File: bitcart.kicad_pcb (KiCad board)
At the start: 4 copper layers, 110 x 100 mm, 125 parts, among them J1 USB_OTG, J10 Conn_02x03_Odd_Even, J12 0455580003, J13 Hashboard0, J14 Hashboard1, J15 Hashboard2, J16 0353180420, J17 0353180420, J18 0353180420, J19 0353180420, J2 690-008-221-904, J3 61900411021, J4 61900411021, J5 61900411021, J6 61900411021, J7 Conn_01x22, J8 Conn_01x02, J9 THD-20-R, Q1 DMP3013SFV-7, U1 FSUSB42MUX, U10 PCA9546ARGVR, U2 USB2514B-I/M2, U3 TPD4EUSB30, U4 AP22653W6, U5 EMC2305-1-AP-TR, U6 74LVC1G07SE-7, U7 MagJack-A70-112-331N126, U9 AP64501SP-13, Y1 24MHz

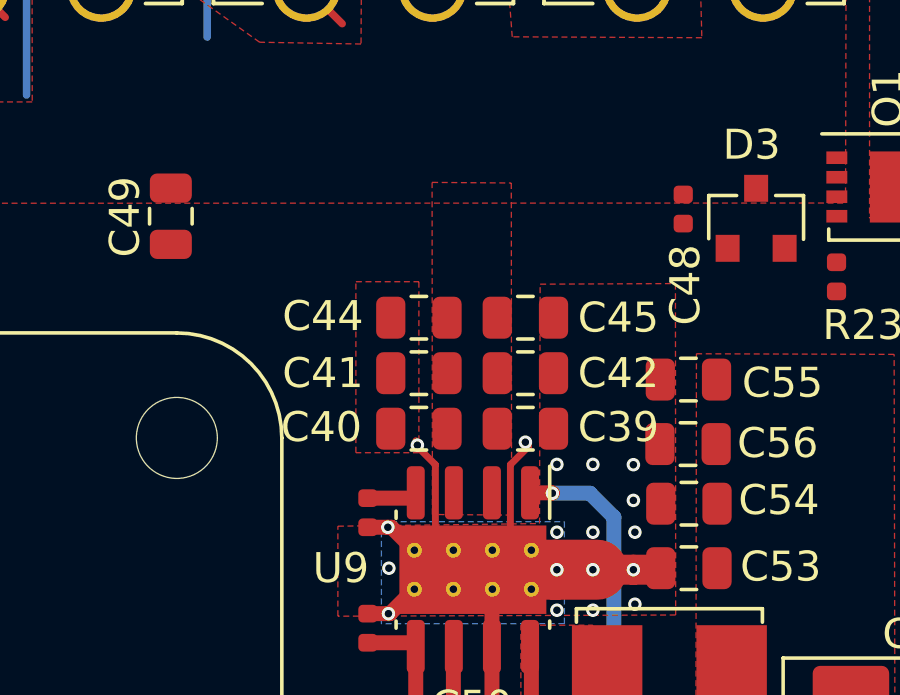
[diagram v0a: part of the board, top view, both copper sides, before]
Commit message: more placement
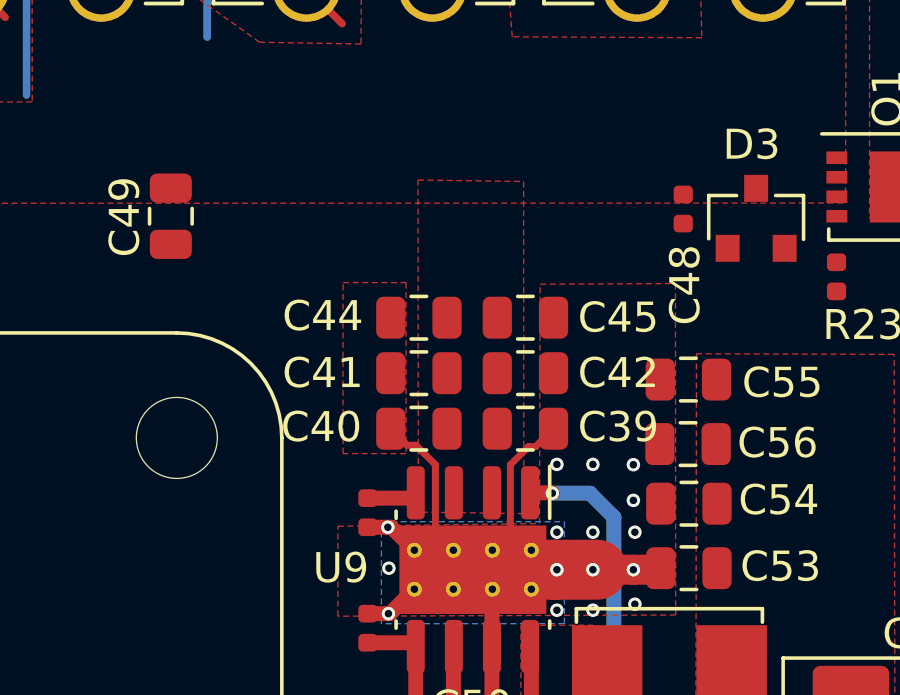
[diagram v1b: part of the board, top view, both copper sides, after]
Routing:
- net GND: track 172.9 -> 174.7 mm, vias 208 -> 206
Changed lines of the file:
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@@
   (segment (start 124.47 108.5) (end 124.47 107.8) (width 0.2) (layer "F.Cu") (net 1))
   (segment (start 117.27 105.4) (end 117.27 104.71001) (width 0.2) (layer "F.Cu") (net 1))
+  (segment (start 157.688553 73.792422) (end 157.926053 73.792422) (width 0.23) (layer "F.Cu") (net 1))
   (segment (start 116.07 105.42) (end 116.07 106.1) (width 0.2) (layer "F.Cu") (net 1))
   (segment (start 113.09 39.66) (end 114.1975 39.66) (width 0.25) (layer "F.Cu") (net 1))
-  (segment (start 153.938553 73.592422) (end 153.938553 73.742422) (width 0.23) (layer "F.Cu") (net 1))
   (segment (start 122.07 107.81001) (end 122.08001 107.8) (width 0.2) (layer "F.Cu") (net 1))
   (segment (start 157.088553 74.392422) (end 157.088553 76.642422) (width 0.23) (layer "F.Cu") (net 1))
@@
   (segment (start 171.054 109.294) (end 171.485 109.725) (width 0.5) (layer "F.Cu") (net 1))
   (segment (start 175.914 114.818) (end 175.914 112.729) (width 0.5) (layer "F.Cu") (net 1))
+  (segment (start 153.651053 73.742422) (end 153.101053 73.192422) (width 0.23) (layer "F.Cu") (net 1))
   (segment (start 125.27 74.58) (end 125.27 75.1) (width 0.2) (layer "F.Cu") (net 1))
   (segment (start 116.47 72.11137) (end 116.406823 72.174547) (width 0.2) (layer "F.Cu") (net 1))
@@
   (segment (start 120.87 108.5) (end 120.87 108.35) (width 0.2) (layer "F.Cu") (net 1))
   (segment (start 119.27 74.58) (end 119.27 75.4) (width 0.2) (layer "F.Cu") (net 1))
-  (segment (start 157.688553 73.592422) (end 157.688553 73.792422) (width 0.23) (layer "F.Cu") (net 1))
   (segment (start 125.27 74.58) (end 125.27 73.980058) (width 0.2) (layer "F.Cu") (net 1))
   (segment (start 179.635 108.575) (end 179.635 108.0375) (width 0.5) (layer "F.Cu") (net 1))
@@
   (segment (start 175.914 114.818) (end 177.91 116.814) (width 0.5) (layer "F.Cu") (net 1))
   (segment (start 178.31 119.95) (end 177.91 120.35) (width 0.2) (layer "F.Cu") (net 1))
+  (segment (start 157.926053 73.792422) (end 158.526053 73.192422) (width 0.23) (layer "F.Cu") (net 1))
   (segment (start 170.9505 109.294) (end 170.9505 110.214474) (width 1) (layer "F.Cu") (net 1))
   (segment (start 178.31 119.55) (end 178.31 119.95) (width 0.2) (layer "F.Cu") (net 1))
@@
   (segment (start 124.45999 105.41001) (end 124.45999 106.1) (width 0.2) (layer "F.Cu") (net 1))
   (segment (start 114.87 108.5) (end 114.87 107.8) (width 0.2) (layer "F.Cu") (net 1))
+  (segment (start 153.938553 73.742422) (end 153.651053 73.742422) (width 0.23) (layer "F.Cu") (net 1))
   (segment (start 120.87 107.8) (end 120.77 107.7) (width 0.13) (layer "F.Cu") (net 1))
   (segment (start 128.07 74.58) (end 128.07 73.9) (width 0.2) (layer "F.Cu") (net 1))
@@
   (via (at 126.88001 104.699345) (size 0.45) (drill 0.25) (layers "F.Cu" "B.Cu") (net 1))
   (via (at 186.2 43.985) (size 0.8) (drill 0.4) (layers "F.Cu" "B.Cu") (free) (net 1))
-  (via (at 157.588553 73.642422) (size 0.45) (drill 0.25) (layers "F.Cu" "B.Cu") (net 1))
   (via (at 110.635 123.08) (size 0.45) (drill 0.25) (layers "F.Cu" "B.Cu") (net 1))
   (via (at 177.91 120.35) (size 0.45) (drill 0.25) (layers "F.Cu" "B.Cu") (net 1))
@@
   (via (at 99.885 128.43) (size 0.45) (drill 0.25) (layers "F.Cu" "B.Cu") (net 1))
   (via (at 186.2 53.09) (size 0.8) (drill 0.4) (layers "F.Cu" "B.Cu") (free) (net 1))
-  (via (at 153.988553 73.742422) (size 0.45) (drill 0.25) (layers "F.Cu" "B.Cu") (net 1))
   (via (at 125.69 109.29) (size 0.45) (drill 0.25) (layers "F.Cu" "B.Cu") (net 1))
   (via (at 129.47 75.4) (size 0.45) (drill 0.25) (layers "F.Cu" "B.Cu") (net 1))
@@
     (polygon
       (pts
-        (xy 154.478553 64.982422)
-        (xy 157.118553 65.002422)
-        (xy 157.128553 76.072422)
-        (xy 154.488553 76.052422)
+        (xy 154.008553 64.902422)
+        (xy 157.528553 64.952422)
+        (xy 157.538553 76.022422)
+        (xy 154.018553 75.972422)
       )
     )
@@
     (polygon
       (pts
-        (xy 151.938553 68.292422)
-        (xy 154.038553 68.292422)
-        (xy 154.038553 73.992422)
-        (xy 151.938553 73.992422)
+        (xy 151.51 68.322422)
+        (xy 153.61 68.322422)
+        (xy 153.61 74.022422)
+        (xy 151.51 74.022422)
       )
     )
